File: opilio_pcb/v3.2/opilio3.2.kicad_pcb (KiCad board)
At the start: 4 copper layers, 80 x 40 mm, 89 parts, among them J1 Screw_Terminal_01x02, J2 Conn_01x02_Male, J3 USB_B_Micro, J4 Program, J5 Conn_01x02_Male, Q1 HSBA3048, Q2 HSBA3048, U1 AMS1117-3.3, U2 SCT51240, U3 SCT51240, U4 USBLC6-2SC6, U5 STM32F103C8T6, Y1 YSX531SL 8MHz, Y2 YST310S 32.768KHz

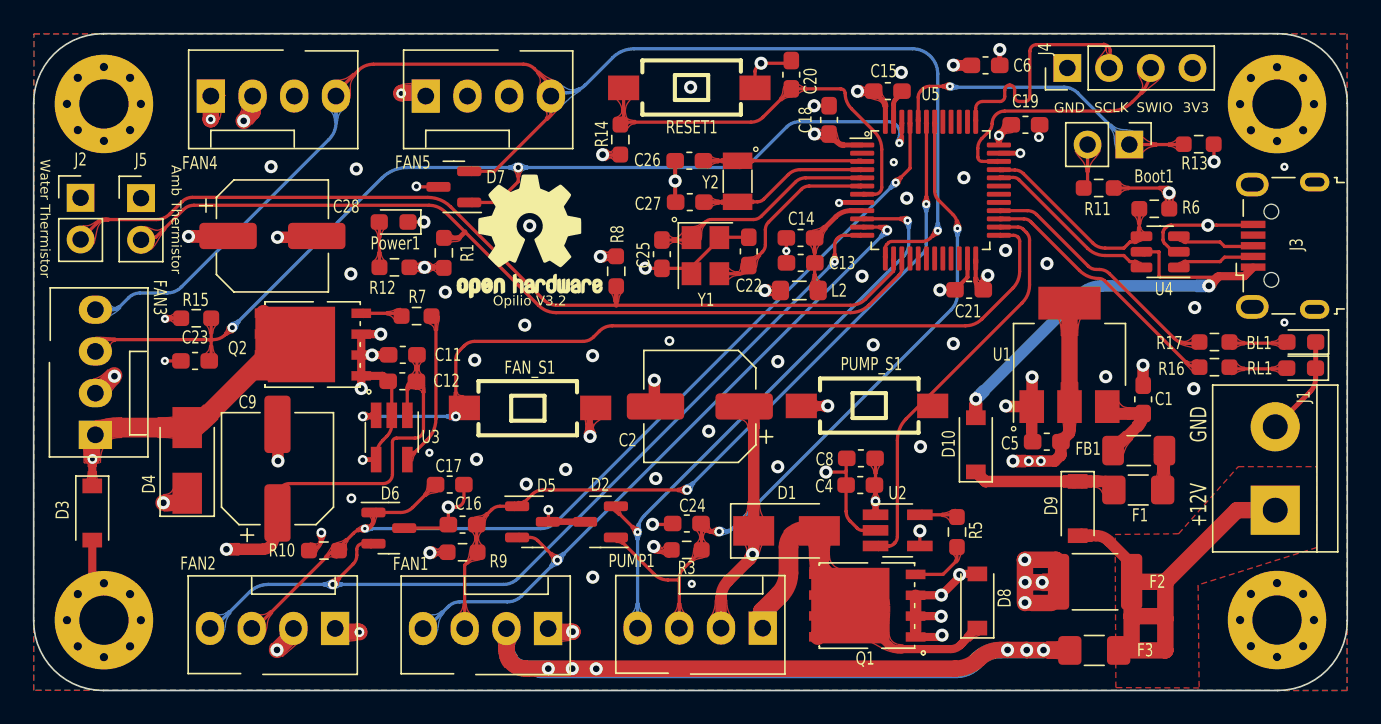
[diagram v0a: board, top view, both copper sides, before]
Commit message: cleanup
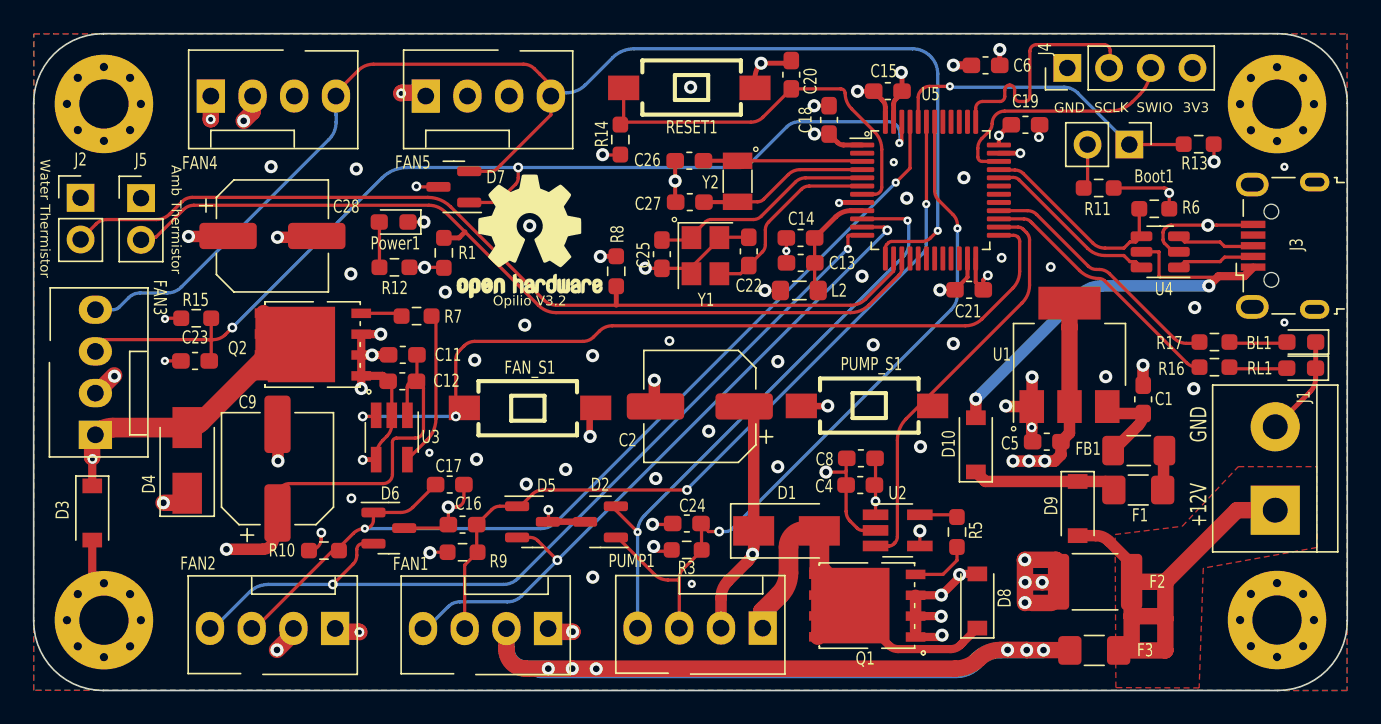
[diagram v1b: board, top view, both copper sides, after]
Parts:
- R5, R7: value 220 -> 24R
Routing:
- net GND: track 102.6 -> 105.6 mm, vias 70 -> 71

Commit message: pcb update
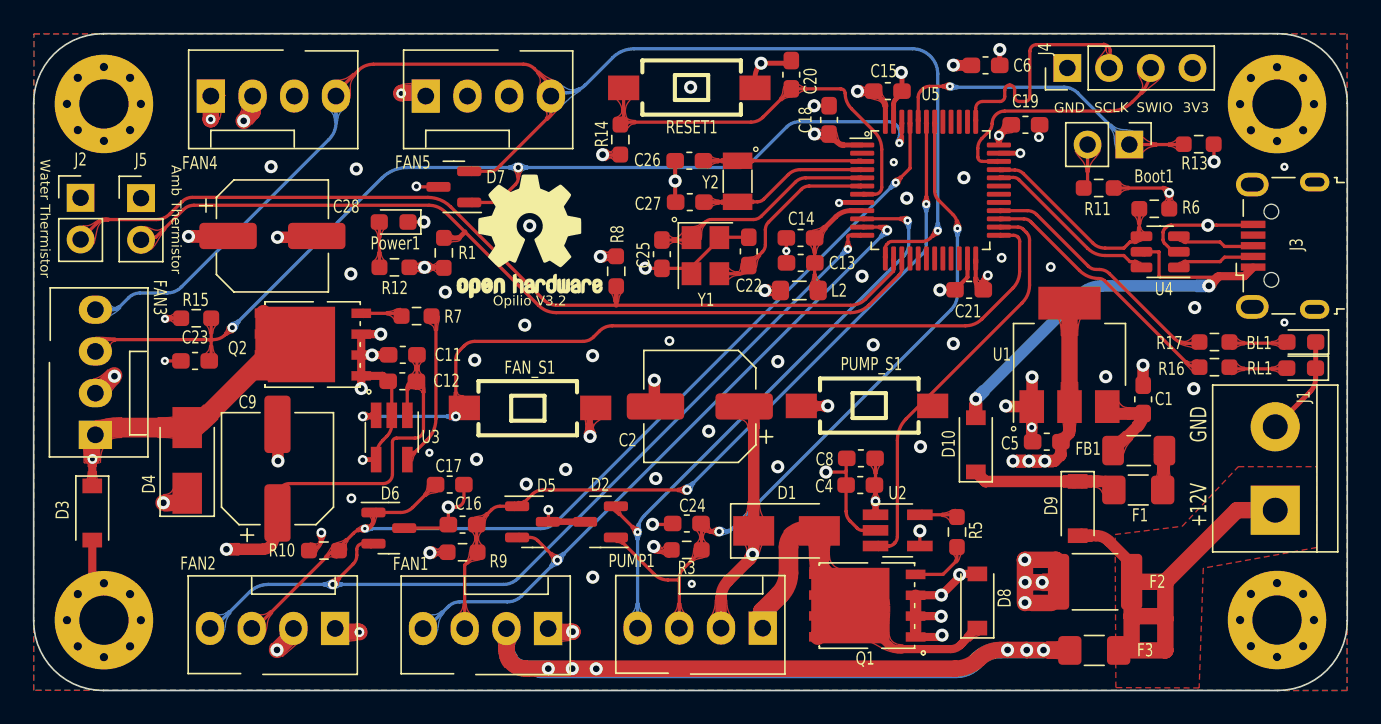
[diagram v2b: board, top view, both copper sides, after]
